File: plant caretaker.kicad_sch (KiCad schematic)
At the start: 1 part, among them U4 ESP32-C3

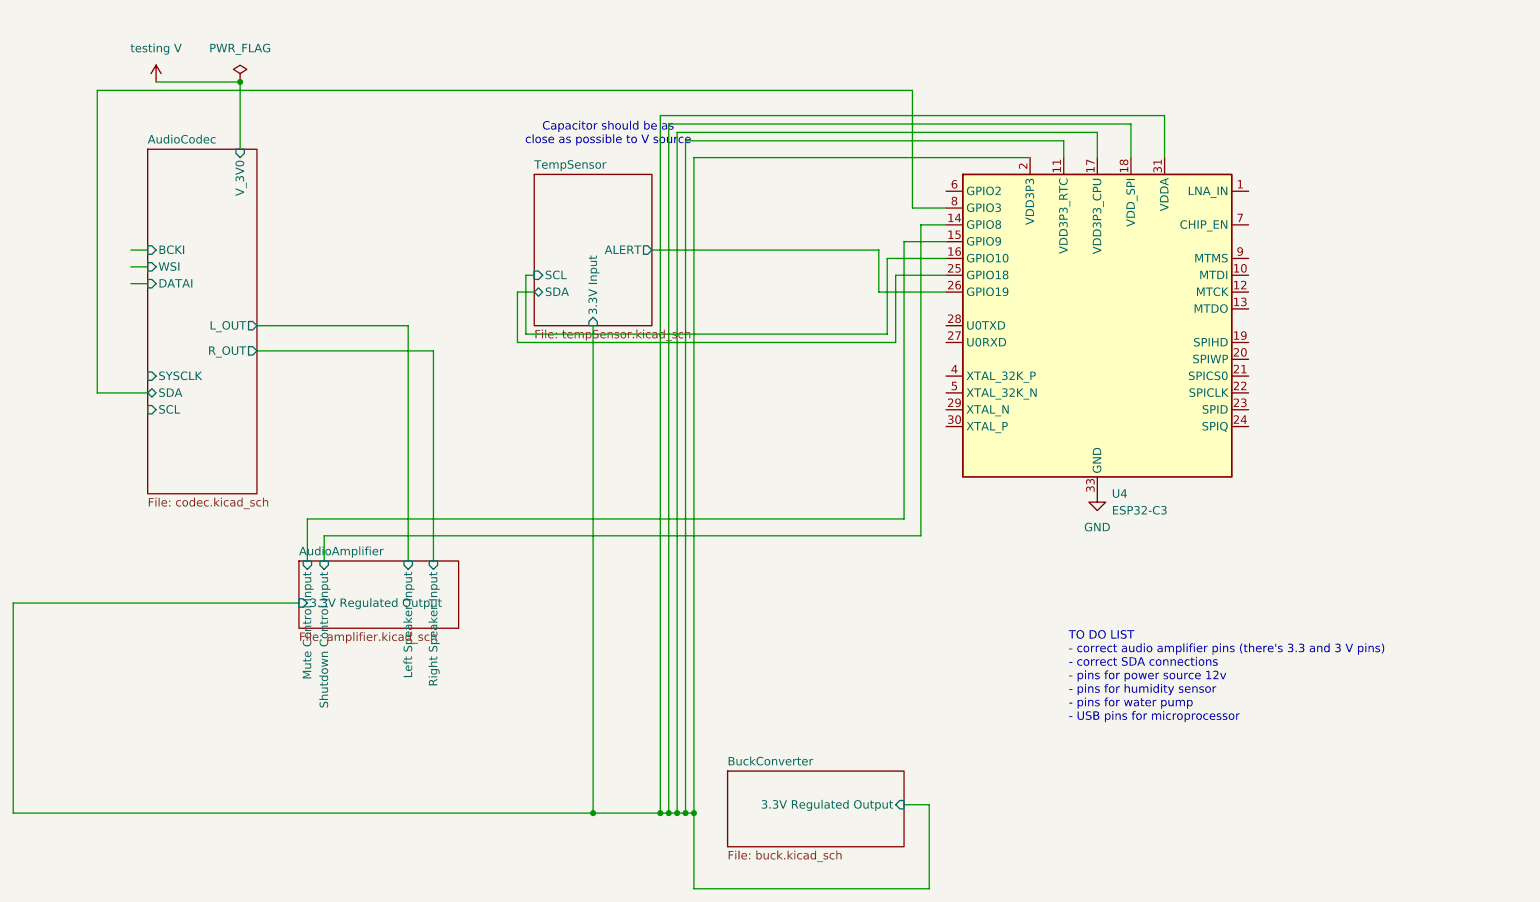
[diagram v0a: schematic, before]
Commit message: Cleanup, sorting, adding external parts
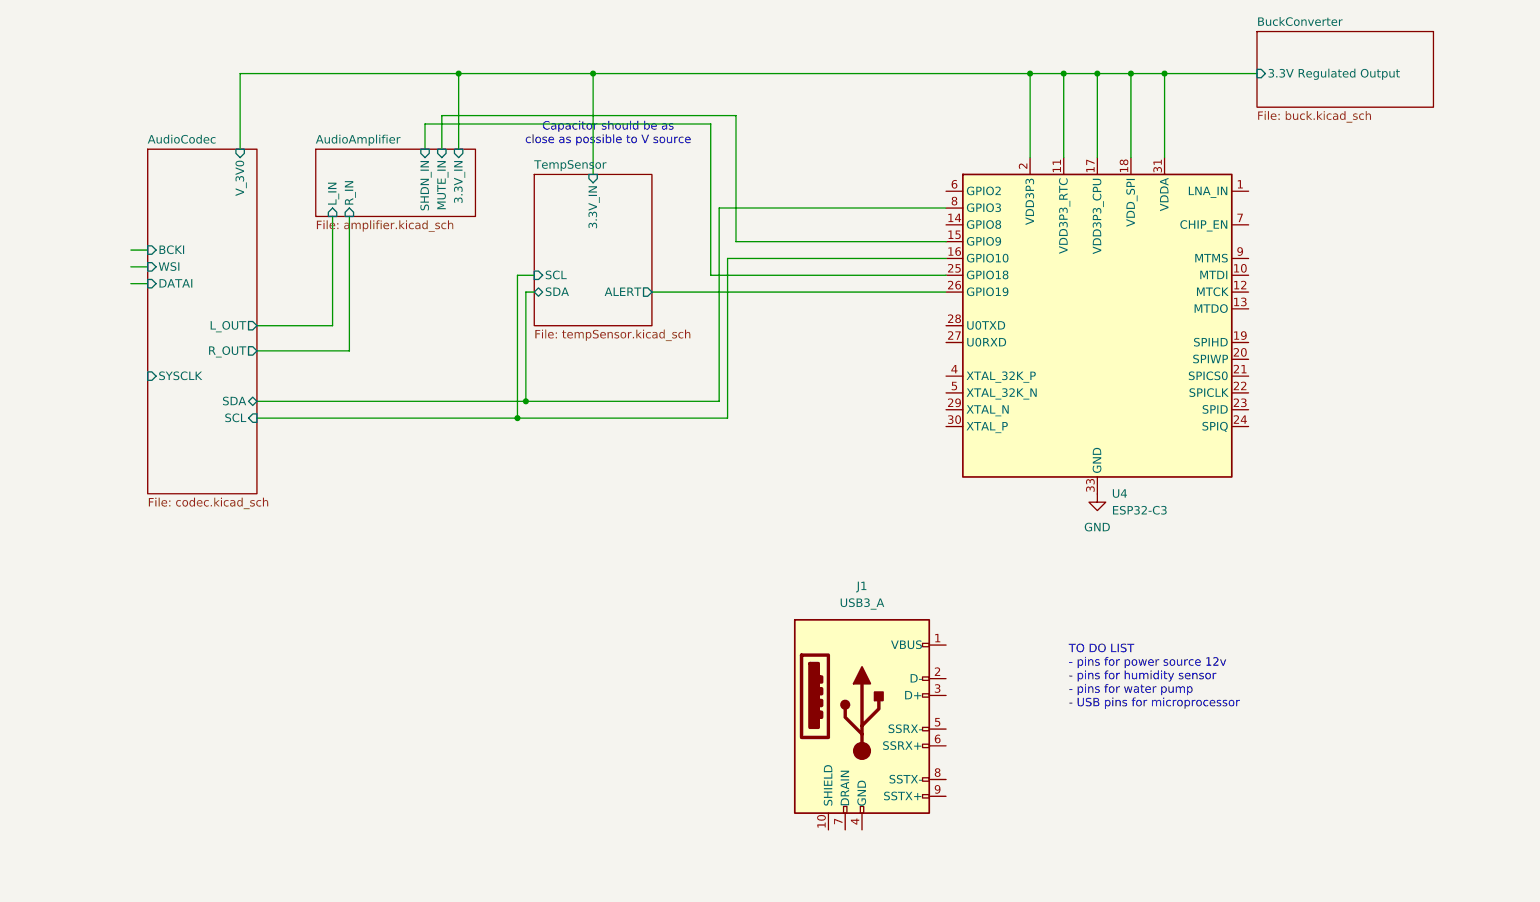
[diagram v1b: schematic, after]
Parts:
- added J1: USB3_A, symbol Connector:USB3_A
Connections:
- net TempSensor/SCL is gone; now on net AudioCodec/SCL: U4.16 (GPIO10)
- net AudioAmplifier/3.3V Regulated Output renamed AudioAmplifier/3.3V_IN
- net AudioAmplifier/Mute Control Input renamed AudioAmplifier/MUTE_IN
- net AudioAmplifier/Shutdown Control Input: no longer names the net of U4.14 (GPIO8)
- net TempSensor/SDA renamed AudioAmplifier/SHDN_IN
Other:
- sheet AudioAmplifier ports: added 3.3V_IN, L_IN, MUTE_IN, R_IN, SHDN_IN; removed 3.3V Regulated Output, Left Speaker Input, Mute Control Input, Right Speaker Input, Shutdown Control Input
- sheet TempSensor ports: added 3.3V_IN; removed 3.3V Input
- note added: "TO DO LIST - pins for power source 12v - pins for humidity sensor - pins for water pump - USB pins for microprocessor"
- note removed: "TO DO LIST - correct audio amplifier pins (there's 3.3 and 3 V pins) - correct SDA connections - pins for power source 12v - pins for humidity sensor - pins for water pump - USB pins for microprocessor"
